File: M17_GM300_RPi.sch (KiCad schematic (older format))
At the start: 46 parts, among them J1 RJ45, J2 DB9_Female, J3 RPi_SND, J4 Conn_01x20_Female, J5 Conn_01x20_Female, J6 Conn_01x02_Female, Q1 BSS123, Q2 BSS123, Q3 BSS123, U1 4066, U2 LM386, U3 MCP6001U

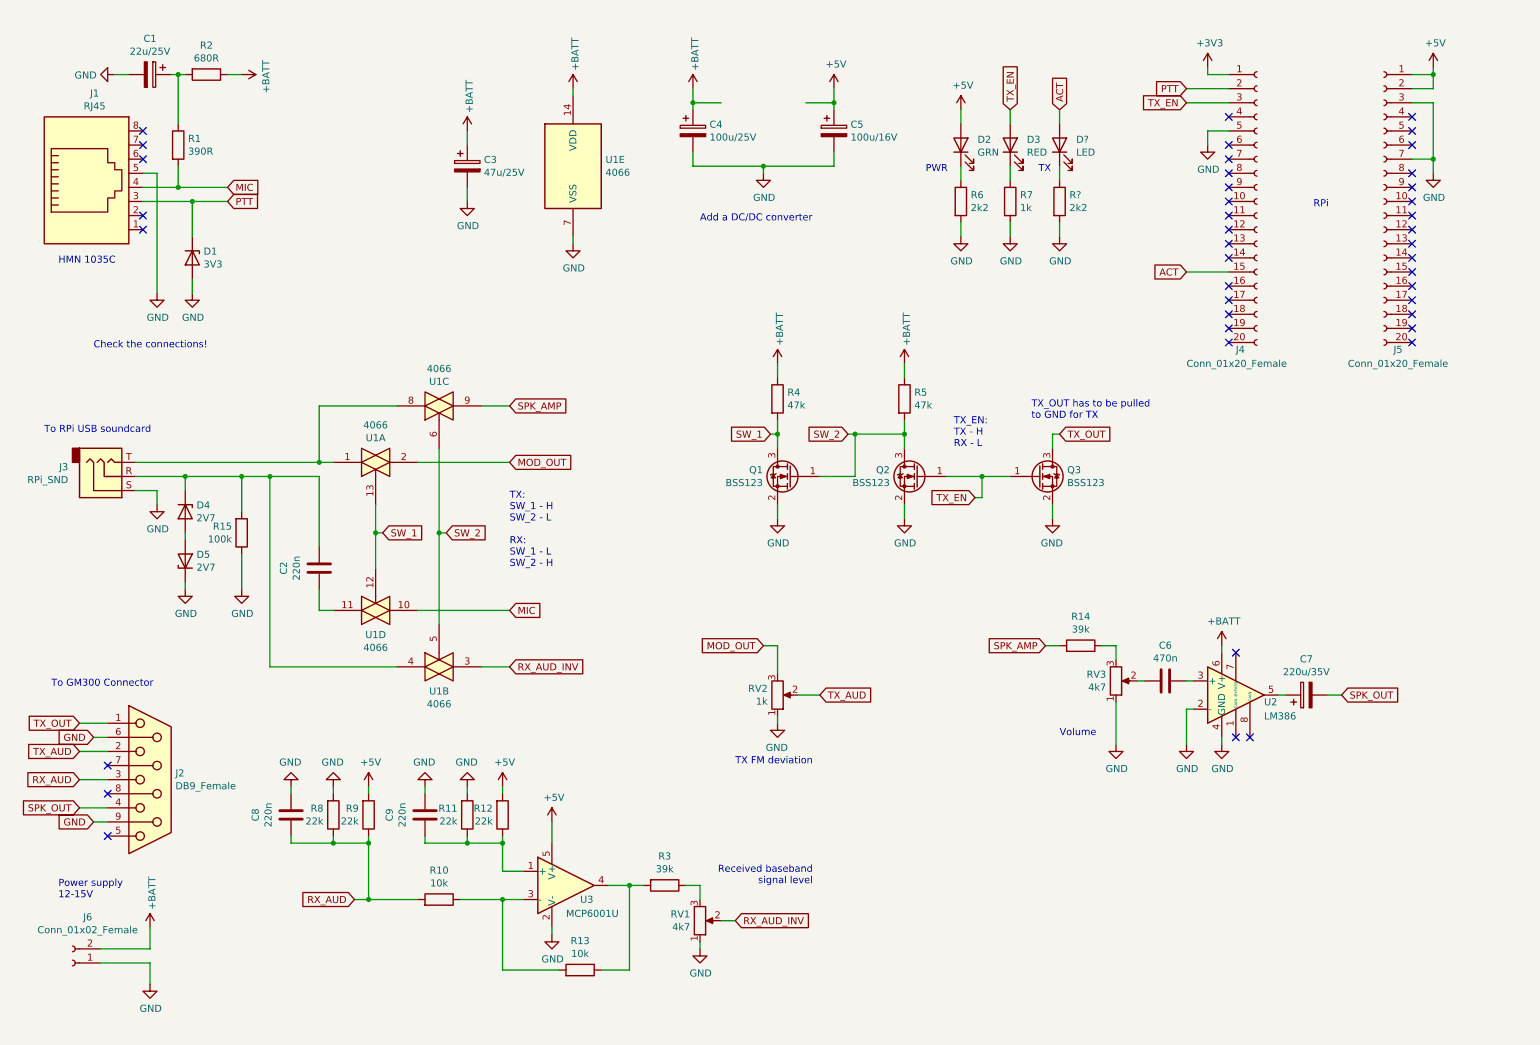
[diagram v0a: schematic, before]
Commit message: redraw
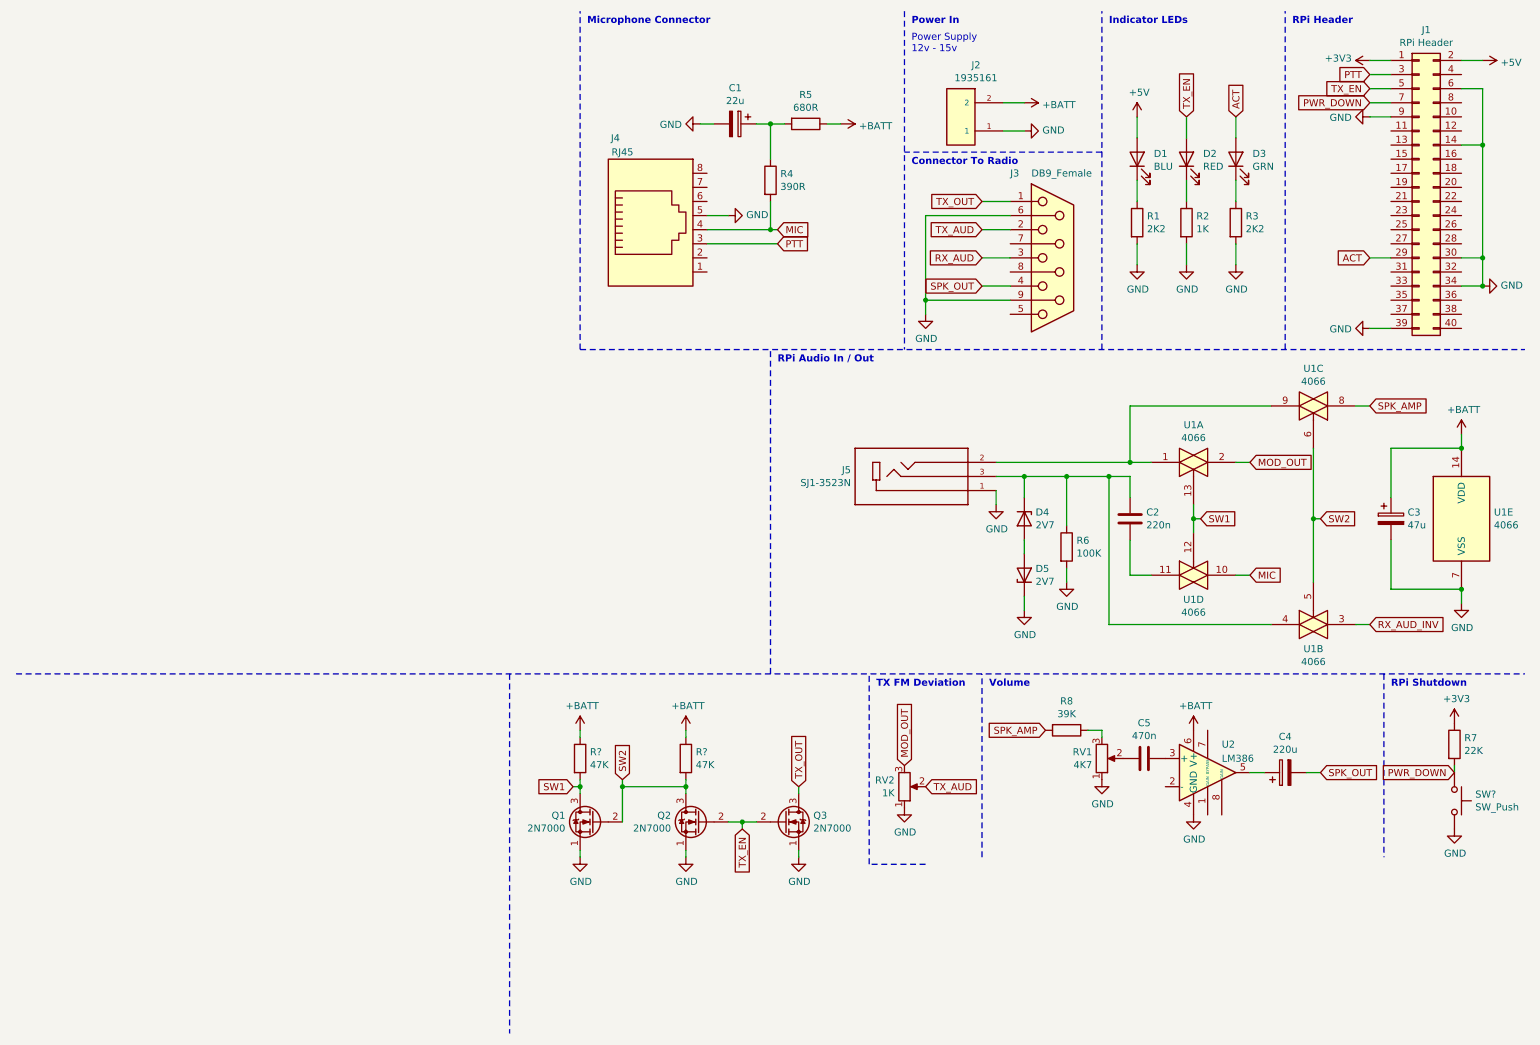
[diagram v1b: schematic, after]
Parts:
- removed C5: 100u/16V, symbol Device:C_Polarized
- removed C6: 470n, symbol Device:C
- removed C7: 220u/35V, symbol Device:C_Polarized
- removed C8, C9: 220n, symbol Device:C
- removed D1: 3V3, symbol Device:D_Zener
- removed D?: LED, symbol Device:LED
- removed J1: RJ45, Connector_RJ:RJ45_Amphenol_RJHSE5380, symbol Connector:8P8C
- removed J2: DB9_Female, symbol Connector:DB9_Female
- removed J3: RPi_SND, symbol Connector:AudioJack3
- removed J4, J5: Conn_01x20_Female, symbol Connector:Conn_01x20_Female
- removed J6: Conn_01x02_Female, symbol Connector:Conn_01x02_Female
- removed Q1, Q2, Q3: BSS123, Package_TO_SOT_SMD:SOT-23, symbol Transistor_FET:BSS123
- removed R10, R13: 10k, symbol Device:R
- removed R11, R12, R9: 22k, symbol Device:R
- removed R14: 39k, symbol Device:R
- removed R15: 100k, symbol Device:R
- removed R?: 2k2, symbol Device:R
- removed RV3: 4k7, symbol Device:R_Potentiometer
- removed U3: MCP6001U, symbol Amplifier_Operational:MCP6001U
- added C5: 470n, Capacitor_THT:C_Disc_D5.0mm_W2.5mm_P5.00mm, symbol Device:C
- added D1: BLU, LED_THT:LED_D3.0mm, symbol Device:LED
- added J1: RPi Header, Connector_PinSocket_2.54mm:PinSocket_2x20_P2.54mm_Vertical, symbol Connector_Generic:Conn_02x20_Odd_Even
- added J2: 1935161, PHOENIX_1935161, symbol 1935161:1935161
- added J3: DB9_Female, Connector_Dsub:DSUB-9_Female_Horizontal_P2.77x2.84mm_EdgePinOffset4.94mm_Housed_MountingHolesOffset7.48mm, symbol Connector:DB9_Female
- added J4: RJ45, Connector_RJ:RJ45_Amphenol_54602-x08_Horizontal, symbol Connector:RJ45
- added J5: SJ1-3523N, CUI_SJ1-3523N, symbol SJ1-3523N:SJ1-3523N
- added Q1, Q2, Q3: 2N7000, Package_TO_SOT_THT:TO-92_HandSolder, symbol Transistor_FET:2N7000
- added R? (x2): 47K, Resistor_THT:R_Axial_DIN0207_L6.3mm_D2.5mm_P7.62mm_Horizontal, symbol Device:R
- added SW?: SW_Push, symbol Switch:SW_Push
- C1: value 22u/25V -> 22u; footprint (none) -> Capacitor_THT:CP_Radial_D8.0mm_P5.00mm
- C2: footprint (none) -> Capacitor_THT:C_Disc_D5.0mm_W2.5mm_P5.00mm
- C3: value 47u/25V -> 47u; footprint (none) -> Capacitor_THT:CP_Radial_D8.0mm_P5.00mm
- C4: value 100u/25V -> 220u; footprint (none) -> Capacitor_THT:CP_Radial_D8.0mm_P5.00mm
- D2: value GRN -> RED; footprint (none) -> LED_THT:LED_D3.0mm
- D3: value RED -> GRN; footprint (none) -> LED_THT:LED_D3.0mm
- R1: value 390R -> 2K2; footprint (none) -> Resistor_THT:R_Axial_DIN0207_L6.3mm_D2.5mm_P7.62mm_Horizontal
- R2: value 680R -> 1K; footprint (none) -> Resistor_THT:R_Axial_DIN0207_L6.3mm_D2.5mm_P7.62mm_Horizontal
- R3: value 39k -> 2K2; footprint (none) -> Resistor_THT:R_Axial_DIN0207_L6.3mm_D2.5mm_P7.62mm_Horizontal
- R4: value 47k -> 390R; footprint (none) -> Resistor_THT:R_Axial_DIN0207_L6.3mm_D2.5mm_P7.62mm_Horizontal
- R5: value 47k -> 680R; footprint (none) -> Resistor_THT:R_Axial_DIN0207_L6.3mm_D2.5mm_P7.62mm_Horizontal
- R6: value 2k2 -> 100K; footprint (none) -> Resistor_THT:R_Axial_DIN0207_L6.3mm_D2.5mm_P7.62mm_Horizontal
- R7: value 1k -> 22K; footprint (none) -> Resistor_THT:R_Axial_DIN0207_L6.3mm_D2.5mm_P7.62mm_Horizontal
- R8: value 22k -> 39K; footprint (none) -> Resistor_THT:R_Axial_DIN0207_L6.3mm_D2.5mm_P7.62mm_Horizontal
- RV1: value 4k7 -> 4K7
- RV2: value 1k -> 1K
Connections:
- net +3V3: now also R7.1, J1.1 (Pin_1)
- net +5V: now also D1.2 (A), J1.2 (Pin_2); no longer D2.2 (A)
- net +BATT: now also J2.2, R?.1, R?.1; no longer C4.1, R2.1, R4.1
- net ACT: now also D3.2 (A), J1.29 (Pin_29)
- net GND: now also R1.2, R2.2, R3.2, J1.14 (Pin_14), J1.30 (Pin_30), J1.34 (Pin_34), J1.39 (Pin_39), J1.6 (Pin_6), J1.9 (Pin_9), J2.1, J3.6, J3.9, J4.5, J5.1, Q1.1 (S), Q2.1 (S), Q3.1 (S), SW?.2; no longer C4.2, R7.2, R8.2, U2.2 (-)
- net MIC: now also R4.2, J4.4; no longer R1.2
- net PTT: now also J1.3 (Pin_3), J4.3
- net RX_AUD: now also J3.3; no longer R8.1
- net RX_AUD_INV: no longer RV1.2
- net SPK_AMP: now also R8.2, U1.8; no longer U1.9
- net SPK_OUT: now also C4.2, J3.4
- net TX_AUD: now also J3.2
- net TX_EN: now also D2.2 (A), J1.5 (Pin_5), Q2.2 (G), Q3.2 (G); no longer D3.2 (A)
- net TX_OUT: now also J3.1, Q3.3 (D)
- net at U1.1: now also U1.9, J5.2; no longer U1.8
- net at C2.1, D4.1 (K), U1.4: now also R6.1, J5.3
- net at R3.1: now also D3.1 (K); no longer RV1.3
- net at U2.3 (+): now also C5.1
- net at U2.5: now also C4.1
- net at D2.1 (K): now also R2.1; no longer R6.1
- net SW_1 renamed SW1
- net SW1: now also Q1.3 (D), R?.2; no longer R4.2
- net SW_2 renamed SW2
- net SW2: now also Q1.2 (G), Q2.3 (D), R?.2; no longer R5.2
- new net: D1.1 (K), R1.1
- new net: C1.1, R4.1, R5.2
- new net: C5.2, RV1.2
- new net: R8.1, RV1.3
- new net PWR_DOWN: J1.7 (Pin_7), R7.2, SW?.1
- no-connect marks 42 -> 0
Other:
- note added: "Connector To Radio"
- note added: "Indicator LEDs"
- note added: "Microphone Connector"
- note added: "Power In"
- note added: "Power Supply\n12v - 15v"
- note added: "RPi Audio In / Out"
- note added: "RPi Header"
- note added: "RPi Shutdown"
- note added: "TX FM Deviation"
- note removed: "Add a DC/DC converter"
- note removed: "Check the connections!"
- note removed: "HMN 1035C"
- note removed: "PWR"
- note removed: "Power supply\n12-15V"
- note removed: "RPi"
- note removed: "Received baseband\nsignal level"
- note removed: "TX"
- note removed: "TX FM deviation"
- note removed: "TX:\nSW_1 - H\nSW_2 - L\n\nRX:\nSW_1 - L\nSW_2 - H"
- note removed: "TX_EN:\nTX - H\nRX - L"
- note removed: "TX_OUT has to be pulled\nto GND for TX"
- note removed: "To GM300 Connector"
- note removed: "To RPi USB soundcard"

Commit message: little things
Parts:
- C1, C3, C4: symbol Device:C_Polarized -> M17_GM300_RPi-rescue:C_Polarized-Device
- RV1, RV2: symbol Device:R_Potentiometer -> M17_GM300_RPi-rescue:R_Potentiometer-Device
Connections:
- net +5V: now also J1.4 (Pin_4)
- no-connect marks 0 -> 27
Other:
- note added: "TRX Switch"
- note added: "TX_EN\nTX - H\nRX - L"
- note added: "TX_OUT is pulled\nto GND for TX"
